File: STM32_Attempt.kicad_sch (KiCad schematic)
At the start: 94 parts, among them J1 Conn_01x04_Male, J2 Conn_01x04_Male, J3 Conn_01x04_Male, J4 Conn_01x04_Male, J5 USB_B_Micro, J6 Conn_01x02, SW1 SW_SPDT, U1 AMS1117-3.3, U2 STM32F103C8T6, Y1 16Mhz

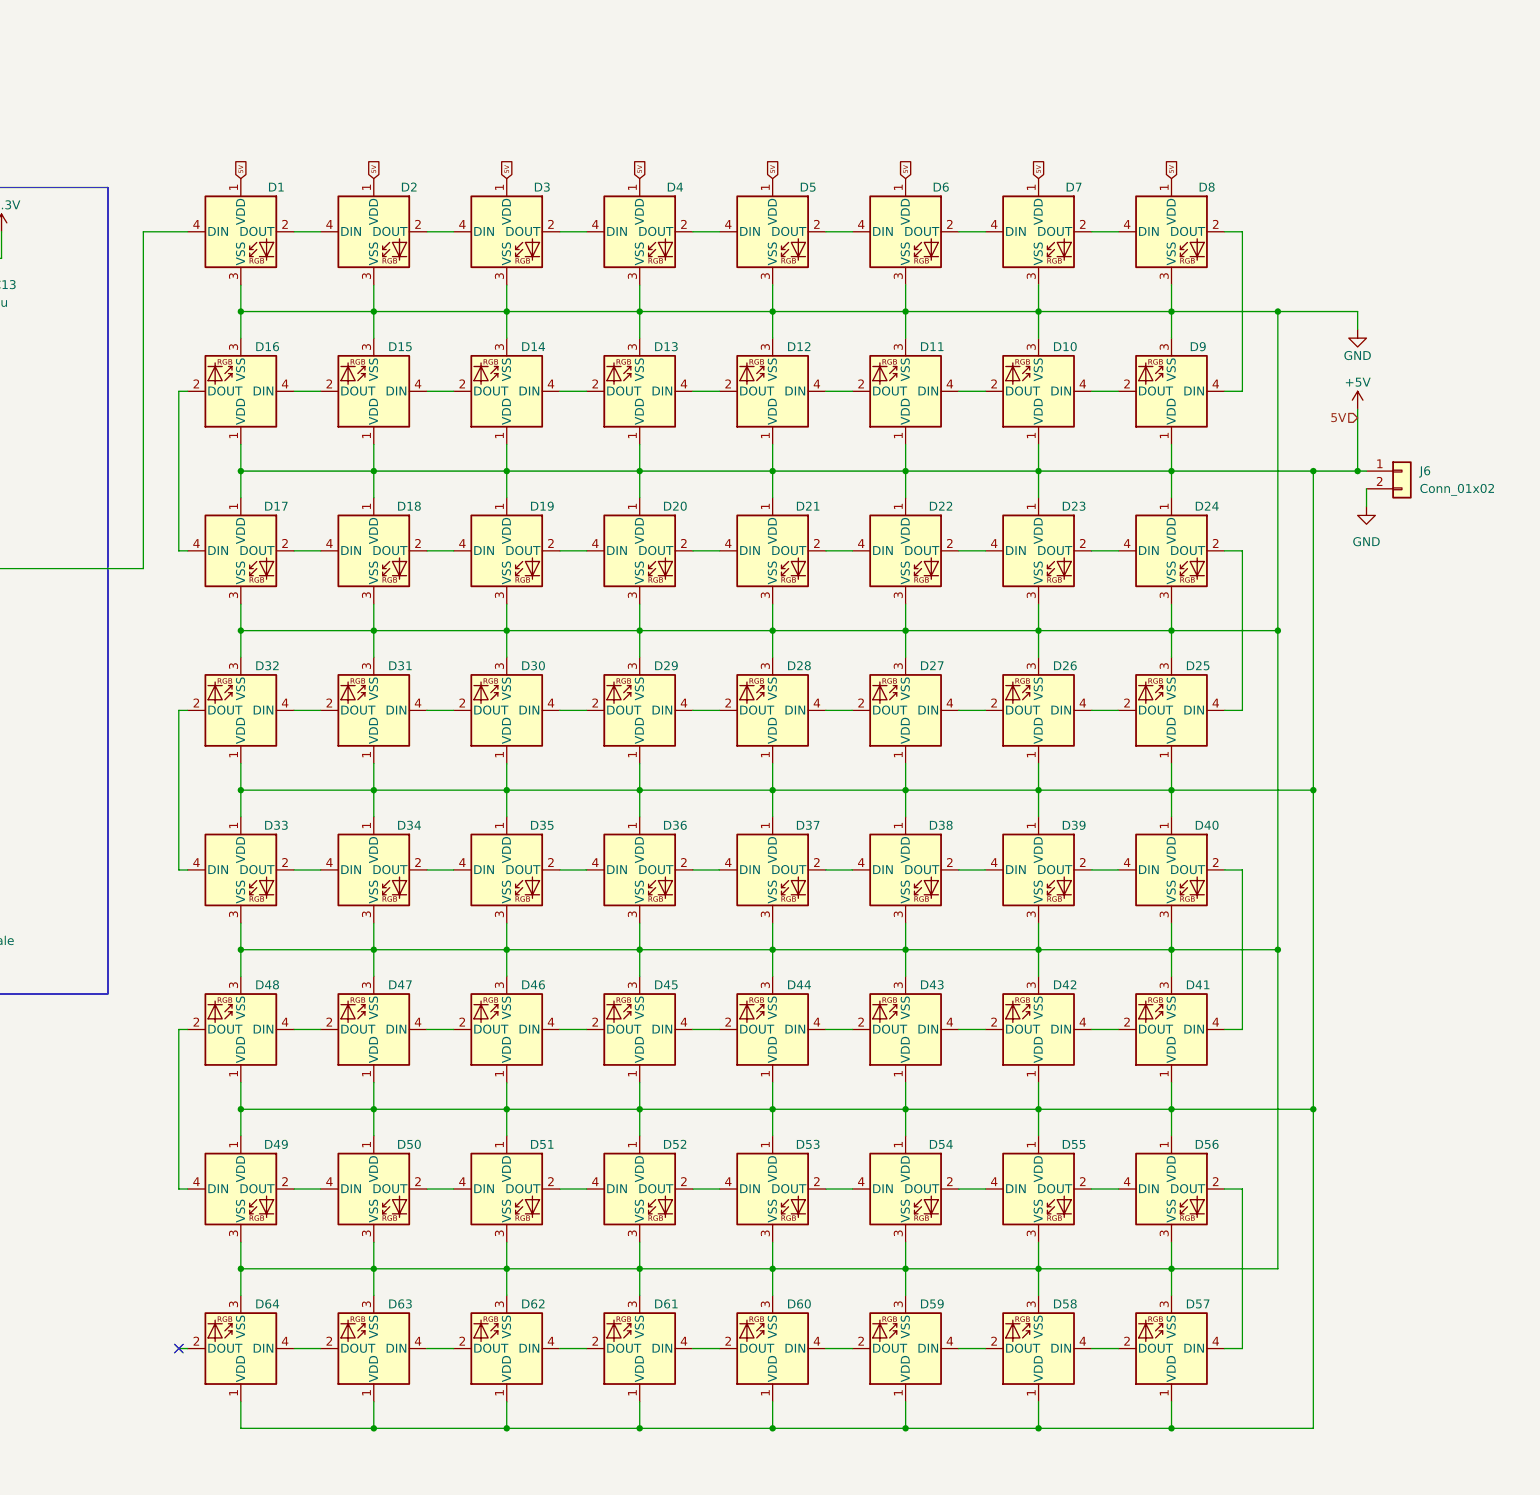
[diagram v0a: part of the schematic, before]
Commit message: 19/10/12 session end
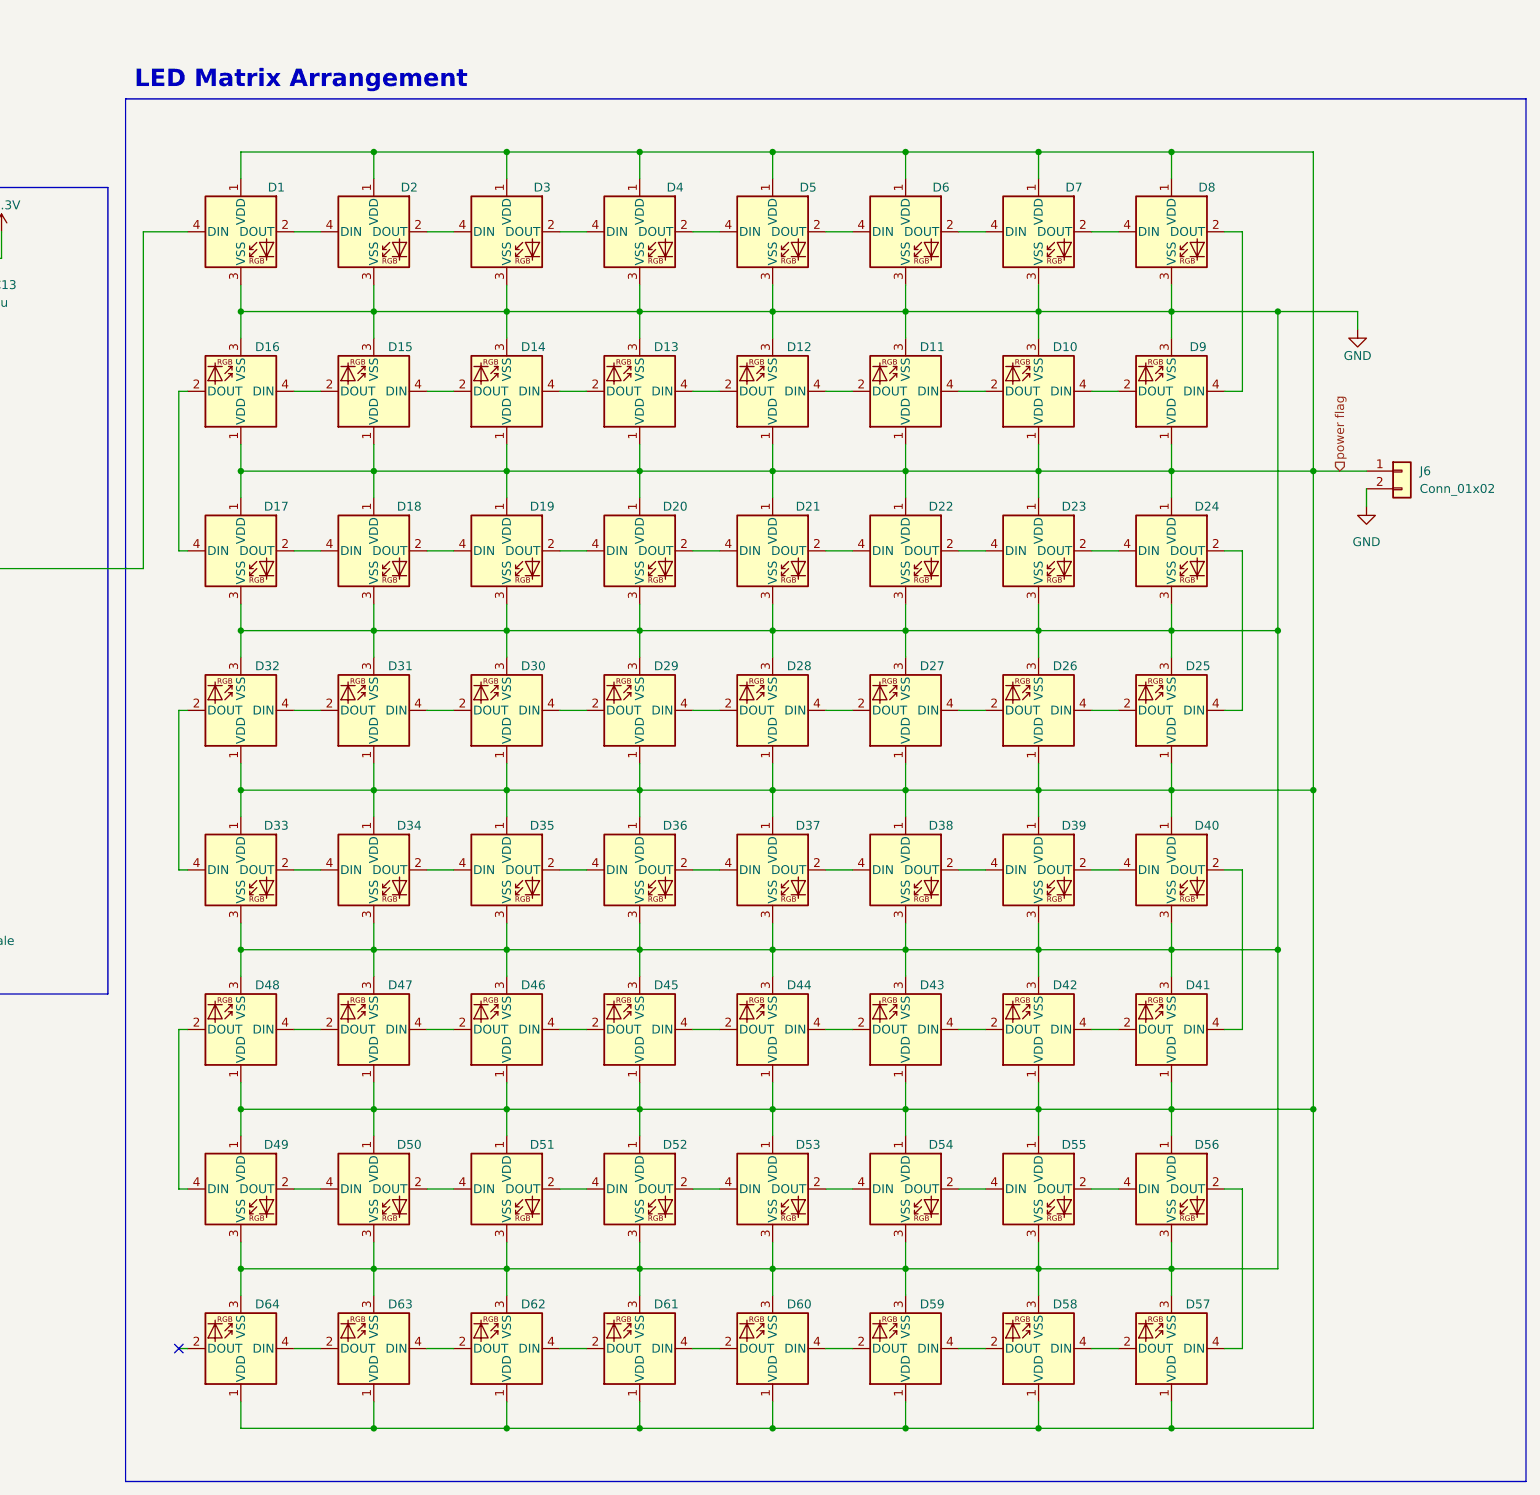
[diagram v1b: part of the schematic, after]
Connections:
- net +5V renamed power flag
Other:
- note added: "LED Matrix Arrangement"
